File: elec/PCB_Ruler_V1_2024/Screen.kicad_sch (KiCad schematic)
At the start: 9 parts, among them SW3 CS1213AGF260, SW4 CS1213AGF260, SW5 CS1213AGF260, SW6 CS1213AGF260, SW7 CS1213AGF260

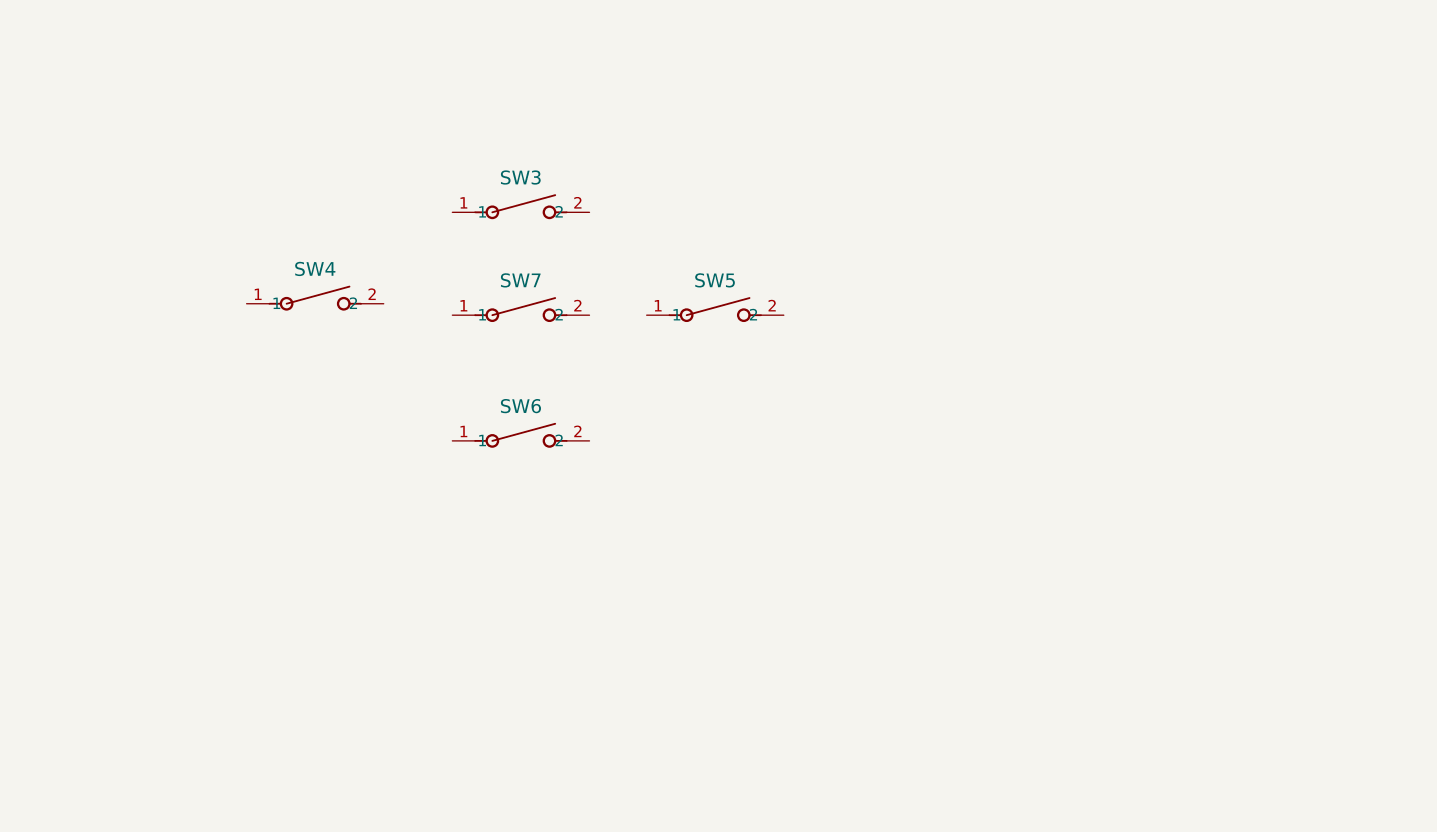
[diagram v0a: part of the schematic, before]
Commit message: protection and Buttons
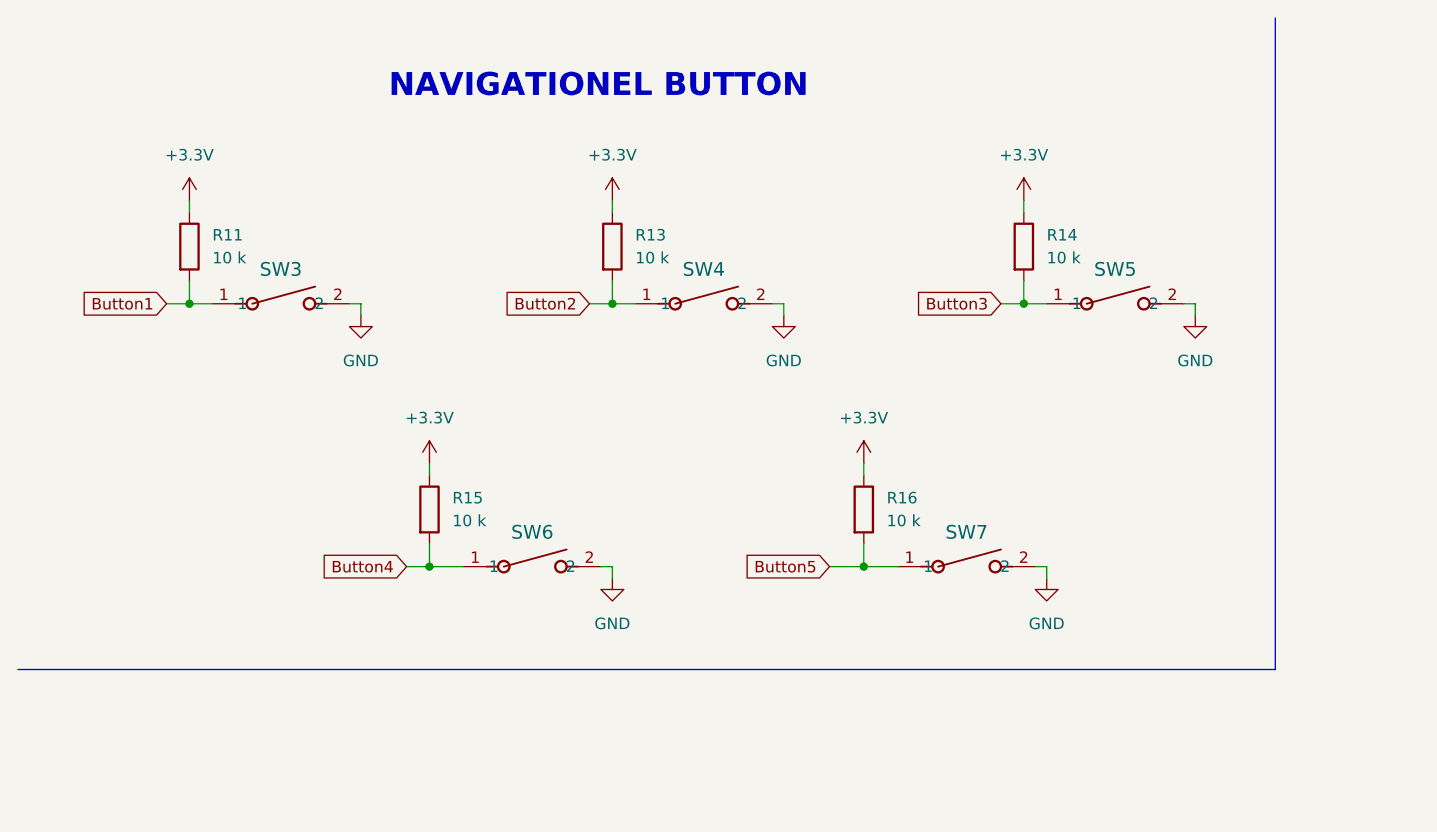
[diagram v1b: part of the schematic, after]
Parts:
- added R11, R13, R14, R15, R16: 10 k, symbol Device:R
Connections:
- net +3.3V: now also R11.1, R13.1, R14.1, R15.1, R16.1
- net GND: now also SW3.2, SW4.2, SW5.2, SW6.2, SW7.2
- net Button3: now reaches SW5.1
- net Button3: now also R14.2
- net Button2: now reaches SW4.1
- net Button2: now also R13.2
- net Button4: now reaches SW6.1
- net Button4: now also R15.2
- net Button1: now reaches SW3.1
- net Button1: now also R11.2
- net Button5: now reaches SW7.1
- net Button5: now also R16.2
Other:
- note added: "NAVIGATIONEL BUTTON"
- moved on the sheet: SW3, SW4, SW5, SW6, SW7
